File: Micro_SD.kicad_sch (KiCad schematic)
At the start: 1 part, among them J1 Micro_SD_Card

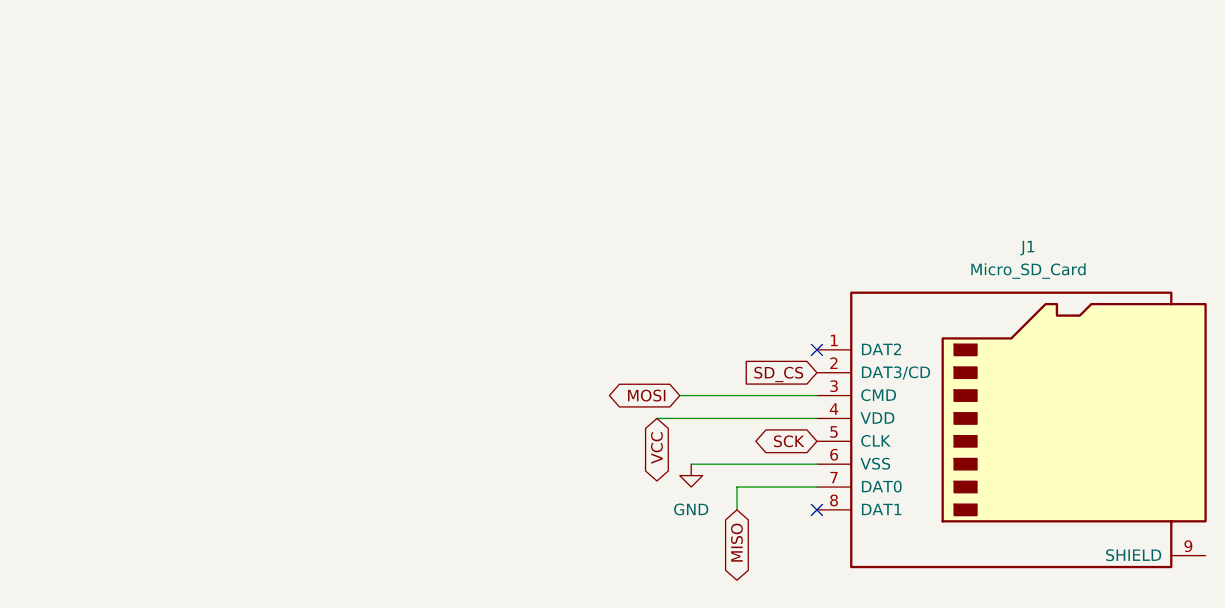
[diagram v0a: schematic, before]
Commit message: Draw basic inital schematic
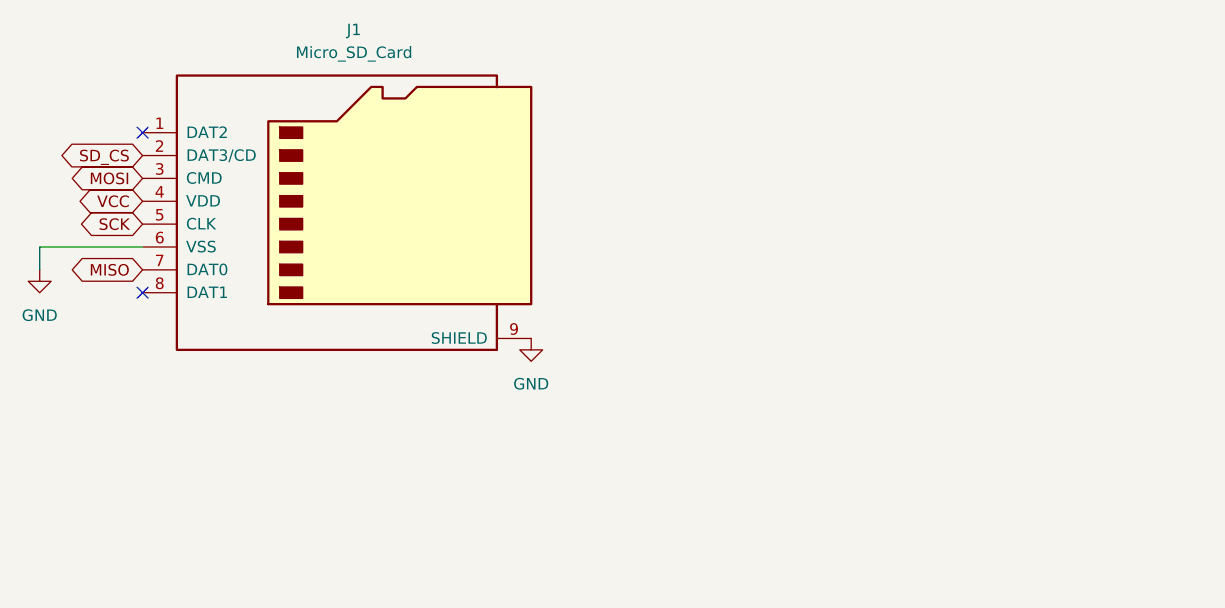
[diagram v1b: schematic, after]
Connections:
- net GND: now also J1.9 (SHIELD)
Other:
- moved on the sheet: J1
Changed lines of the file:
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@@
 	(paper "A4")
 	(no_connect
-		(at 106.68 52.07)
+		(at 31.75 27.94)
 	)
 	(no_connect
-		(at 106.68 69.85)
+		(at 31.75 45.72)
 	)
 	(wire
 		(pts
-			(xy 91.44 57.15) (xy 106.68 57.15)
+			(xy 20.32 40.64) (xy 31.75 40.64)
 		)
 		(stroke
@@
 	(wire
 		(pts
-			(xy 92.71 64.77) (xy 106.68 64.77)
+			(xy 20.32 43.18) (xy 20.32 40.64)
 		)
 		(stroke
@@
 		)
 	)
-	(wire
-		(pts
-			(xy 106.68 67.31) (xy 97.79 67.31)
-		)
-		(stroke
-			(width 0)
-			(type default)
-		)
-	)
-	(wire
-		(pts
-			(xy 88.9 59.69) (xy 106.68 59.69)
-		)
-		(stroke
-			(width 0)
-			(type default)
-		)
-	)
-	(wire
-		(pts
-			(xy 97.79 67.31) (xy 97.79 69.85)
-		)
-		(stroke
-			(width 0)
-			(type default)
-		)
-	)
 	(global_label "MISO"
 		(shape bidirectional)
-		(at 97.79 69.85 270)
-		(fields_autoplaced yes)
-		(effects
-			(font
-				(size 1.27 1.27)
-			)
-			(justify right)
-		)
-		(property "Intersheetrefs" "${INTERSHEET_REFS}"
-			(at 97.79 78.5427 90)
+		(at 31.75 43.18 180)
+		(fields_autoplaced yes)
+		(effects
+			(font
+				(size 1.27 1.27)
+			)
+			(justify right)
+		)
+		(property "Intersheetrefs" "${INTERSHEET_REFS}"
+			(at 23.0573 43.18 0)
 			(effects
 				(font
@@
 	(global_label "MOSI"
 		(shape bidirectional)
-		(at 91.44 57.15 180)
-		(fields_autoplaced yes)
-		(effects
-			(font
-				(size 1.27 1.27)
-			)
-			(justify right)
-		)
-		(property "Intersheetrefs" "${INTERSHEET_REFS}"
-			(at 82.7473 57.15 0)
+		(at 31.75 33.02 180)
+		(fields_autoplaced yes)
+		(effects
+			(font
+				(size 1.27 1.27)
+			)
+			(justify right)
+		)
+		(property "Intersheetrefs" "${INTERSHEET_REFS}"
+			(at 23.0573 33.02 0)
 			(effects
 				(font
@@
 	)
 	(global_label "SD_CS"
-		(shape input)
-		(at 106.68 54.61 180)
-		(fields_autoplaced yes)
-		(effects
-			(font
-				(size 1.27 1.27)
-			)
-			(justify right)
-		)
-		(property "Intersheetrefs" "${INTERSHEET_REFS}"
-			(at 97.7682 54.61 0)
+		(shape bidirectional)
+		(at 31.75 30.48 180)
+		(fields_autoplaced yes)
+		(effects
+			(font
+				(size 1.27 1.27)
+			)
+			(justify right)
+		)
+		(property "Intersheetrefs" "${INTERSHEET_REFS}"
+			(at 21.7269 30.48 0)
 			(effects
 				(font
@@
 	(global_label "VCC"
 		(shape bidirectional)
-		(at 88.9 59.69 270)
-		(fields_autoplaced yes)
-		(effects
-			(font
-				(size 1.27 1.27)
-			)
-			(justify right)
-		)
-		(property "Intersheetrefs" "${INTERSHEET_REFS}"
-			(at 88.9 67.4151 90)
+		(at 31.75 35.56 180)
+		(fields_autoplaced yes)
+		(effects
+			(font
+				(size 1.27 1.27)
+			)
+			(justify right)
+		)
+		(property "Intersheetrefs" "${INTERSHEET_REFS}"
+			(at 24.0249 35.56 0)
 			(effects
 				(font
@@
 	(global_label "SCK"
 		(shape bidirectional)
-		(at 106.68 62.23 180)
-		(fields_autoplaced yes)
-		(effects
-			(font
-				(size 1.27 1.27)
-			)
-			(justify right)
-		)
-		(property "Intersheetrefs" "${INTERSHEET_REFS}"
-			(at 98.834 62.23 0)
+		(at 31.75 38.1 180)
+		(fields_autoplaced yes)
+		(effects
+			(font
+				(size 1.27 1.27)
+			)
+			(justify right)
+		)
+		(property "Intersheetrefs" "${INTERSHEET_REFS}"
+			(at 23.904 38.1 0)
 			(effects
 				(font
@@
 	(symbol
 		(lib_id "Connector:Micro_SD_Card")
-		(at 129.54 59.69 0)
+		(at 54.61 35.56 0)
 		(unit 1)
 		(exclude_from_sim no)
@@
 		(fields_autoplaced yes)
 		(property "Reference" "J1"
-			(at 130.175 40.64 0)
+			(at 55.245 16.51 0)
 			(effects
 				(font
@@
 		)
 		(property "Value" "Micro_SD_Card"
-			(at 130.175 43.18 0)
+			(at 55.245 19.05 0)
 			(effects
 				(font
@@
 		)
 		(property "Footprint" ""
-			(at 158.75 52.07 0)
+			(at 83.82 27.94 0)
 			(effects
 				(font
@@
 		)
 		(property "Datasheet" "https://www.we-online.com/components/products/datasheet/693072010801.pdf"
-			(at 129.54 59.69 0)
+			(at 54.61 35.56 0)
 			(effects
 				(font
@@
 		)
 		(property "Description" "Micro SD Card Socket"
-			(at 129.54 59.69 0)
+			(at 54.61 35.56 0)
 			(effects
 				(font
@@
 	(symbol
 		(lib_id "power:GND")
-		(at 92.71 64.77 0)
+		(at 74.93 50.8 0)
 		(unit 1)
 		(exclude_from_sim no)
@@
 		(dnp no)
 		(fields_autoplaced yes)
-		(property "Reference" "#PWR017"
-			(at 92.71 71.12 0)
+		(property "Reference" "#PWR07"
+			(at 74.93 57.15 0)
 			(effects
 				(font
@@
 		)
 		(property "Value" "GND"
-			(at 92.71 69.85 0)
+			(at 74.93 55.88 0)
 			(effects
 				(font
@@
 		)
 		(property "Footprint" ""
-			(at 92.71 64.77 0)
+			(at 74.93 50.8 0)
 			(effects
 				(font
@@
 		)
 		(property "Datasheet" ""
-			(at 92.71 64.77 0)
+			(at 74.93 50.8 0)
 			(effects
 				(font
@@
 		)
 		(property "Description" "Power symbol creates a global label with name \"GND\" , ground"
-			(at 92.71 64.77 0)
+			(at 74.93 50.8 0)
 			(effects
 				(font
@@
 			(project "plokkskeem"
 				(path "/a526e2f2-17cc-4dbb-8268-7175c0e116d3/2047e8fb-45bc-4387-a87d-c0859c6ee695"
-					(reference "#PWR017")
+					(reference "#PWR07")
 					(unit 1)
 				)
+			)
+		)
+	)
+	(symbol
+		(lib_id "power:GND")
+		(at 20.32 43.18 0)
+		(unit 1)
+		(exclude_from_sim no)
+		(in_bom yes)
+		(on_board yes)
+		(dnp no)
+		(fields_autoplaced yes)
+		(property "Reference" "#PWR06"
+			(at 20.32 49.53 0)
+			(effects
+				(font
+					(size 1.27 1.27)
+				)
+				(hide yes)
+			)
+		)
+		(property "Value" "GND"
+			(at 20.32 48.26 0)
+			(effects
+				(font
+					(size 1.27 1.27)
+				)
+			)
+		)
+		(property "Footprint" ""
+			(at 20.32 43.18 0)
+			(effects
+				(font
+					(size 1.27 1.27)
+				)
+				(hide yes)
+			)
+		)
+		(property "Datasheet" ""
+			(at 20.32 43.18 0)
+			(effects
+				(font
+					(size 1.27 1.27)
+				)
+				(hide yes)
+			)
+		)
+		(property "Description" "Power symbol creates a global label with name \"GND\" , ground"
+			(at 20.32 43.18 0)
+			(effects
+				(font
+					(size 1.27 1.27)
+				)
+				(hide yes)
+			)
+		)
+		(pin "1"
+		)
+		(instances
+			(project "plokkskeem"
+				(path "/a526e2f2-17cc-4dbb-8268-7175c0e116d3/2047e8fb-45bc-4387-a87d-c0859c6ee695"
+					(reference "#PWR06")
+					(unit 1)
+				)

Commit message: viskasin kõik ühele lehele.
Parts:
- removed J1: Micro_SD_Card, symbol Connector:Micro_SD_Card
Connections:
- no-connect marks 2 -> 0
